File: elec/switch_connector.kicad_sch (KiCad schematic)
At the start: 7 parts, among them J3 BM04B-SRSS-TB, Q1 2N7002

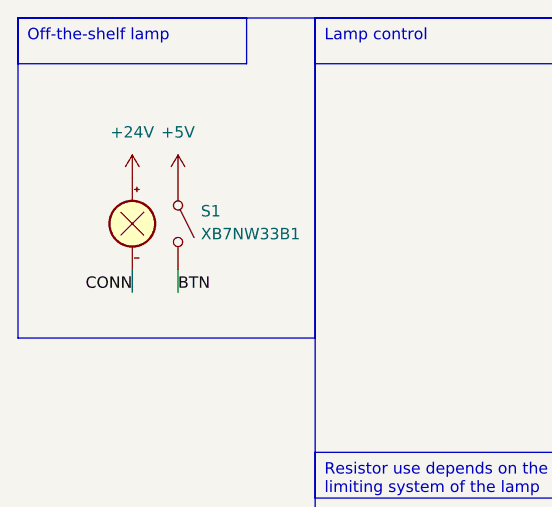
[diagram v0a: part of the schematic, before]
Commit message: dev: updating pcb
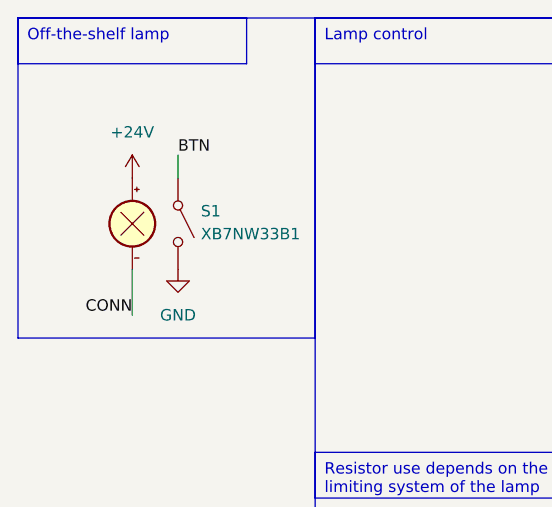
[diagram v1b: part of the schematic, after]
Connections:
- net +5V is gone; now on net BTN: S1.1 (13)
- net BTN: no longer S1.2 (14)
- net GND: now also S1.2 (14)
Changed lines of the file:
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@@
 	(wire
 		(pts
-			(xy 25.4 43.18) (xy 25.4 40.64)
+			(xy 25.4 45.72) (xy 25.4 40.64)
 		)
 		(stroke
@@
 	(wire
 		(pts
-			(xy 30.48 43.18) (xy 30.48 40.64)
+			(xy 30.48 27.94) (xy 30.48 30.48)
 		)
 		(stroke
@@
 	)
 	(label "BTN"
-		(at 30.48 43.18 0)
+		(at 30.48 27.94 0)
 		(fields_autoplaced yes)
 		(effects
@@
 	)
 	(label "CONN"
-		(at 25.4 43.18 180)
+		(at 25.4 45.72 180)
 		(fields_autoplaced yes)
 		(effects
@@
 	)
 	(symbol
+		(lib_id "power:GND")
+		(at 30.48 40.64 0)
+		(unit 1)
+		(exclude_from_sim no)
+		(in_bom yes)
+		(on_board yes)
+		(dnp no)
+		(fields_autoplaced yes)
+		(property "Reference" "#PWR028"
+			(at 30.48 46.99 0)
+			(effects
+				(font
+					(size 1.27 1.27)
+				)
+				(hide yes)
+			)
+		)
+		(property "Value" "GND"
+			(at 30.48 45.72 0)
+			(effects
+				(font
+					(size 1.27 1.27)
+				)
+			)
+		)
+		(property "Footprint" ""
+			(at 30.48 40.64 0)
+			(effects
+				(font
+					(size 1.27 1.27)
+				)
+				(hide yes)
+			)
+		)
+		(property "Datasheet" ""
+			(at 30.48 40.64 0)
+			(effects
+				(font
+					(size 1.27 1.27)
+				)
+				(hide yes)
+			)
+		)
+		(property "Description" "Power symbol creates a global label with name \"GND\" , ground"
+			(at 30.48 40.64 0)
+			(effects
+				(font
+					(size 1.27 1.27)
+				)
+				(hide yes)
+			)
+		)
+		(pin "1"
+		)
+		(instances
+			(project "elec"
+				(path "/9721bce9-01f4-4230-bc1e-748d0303b61d/d1c63f12-a9c6-44fc-aada-0b6e04e33293"
+					(reference "#PWR028")
+					(unit 1)
+				)
+				(path "/9721bce9-01f4-4230-bc1e-748d0303b61d/5ed1a42c-1f8a-456f-aca4-b0ec53e5043f"
+					(reference "#PWR036")
+					(unit 1)
+				)
+				(path "/9721bce9-01f4-4230-bc1e-748d0303b61d/fdf19939-3d9b-4110-9022-c37157a29402"
+					(reference "#PWR044")
+					(unit 1)
+				)
+				(path "/9721bce9-01f4-4230-bc1e-748d0303b61d/37f927af-89ef-4fdd-8956-bca34548d96f"
+					(reference "#PWR052")
+					(unit 1)
+				)
+				(path "/9721bce9-01f4-4230-bc1e-748d0303b61d/986b1860-5bd6-47a5-b66e-b737b7bd0f11"
+					(reference "#PWR060")
+					(unit 1)
+				)
+				(path "/9721bce9-01f4-4230-bc1e-748d0303b61d/eebd9391-916f-49b6-bec7-88d6969a1573"
+					(reference "#PWR068")
+					(unit 1)
+				)
+				(path "/9721bce9-01f4-4230-bc1e-748d0303b61d/d67cbc77-a7b3-4445-bb70-2db77a7feb74"
+					(reference "#PWR076")
+					(unit 1)
+				)
+				(path "/9721bce9-01f4-4230-bc1e-748d0303b61d/3bc99195-9e3c-4290-911f-d629015a354c"
+					(reference "#PWR084")
+					(unit 1)
+				)
+				(path "/9721bce9-01f4-4230-bc1e-748d0303b61d/e3e2ca04-3651-46d9-8ec0-5b3aca5c73d2"
+					(reference "#PWR092")
+					(unit 1)
+				)
+				(path "/9721bce9-01f4-4230-bc1e-748d0303b61d/333f48b8-09d6-4cfc-b48e-393e968338e9"
+					(reference "#PWR0100")
+					(unit 1)
+				)
+			)
+		)
+	)
+	(symbol
 		(lib_id "breakout:XB7NW33B1")
 		(at 30.48 35.56 0)
@@
 					(unit 1)
 				)
-			)
-		)
-	)
-	(symbol
-		(lib_id "power:+5V")
-		(at 30.48 30.48 0)
-		(unit 1)
-		(exclude_from_sim no)
-		(in_bom yes)
-		(on_board yes)
-		(dnp no)
-		(fields_autoplaced yes)
-		(property "Reference" "#PWR028"
-			(at 30.48 34.29 0)
-			(effects
-				(font
-					(size 1.27 1.27)
-				)
-				(hide yes)
-			)
-		)
-		(property "Value" "+5V"
-			(at 30.48 25.4 0)
-			(effects
-				(font
-					(size 1.27 1.27)
-				)
-			)
-		)
-		(property "Footprint" ""
-			(at 30.48 30.48 0)
-			(effects
-				(font
-					(size 1.27 1.27)
-				)
-				(hide yes)
-			)
-		)
-		(property "Datasheet" ""
-			(at 30.48 30.48 0)
-			(effects
-				(font
-					(size 1.27 1.27)
-				)
-				(hide yes)
-			)
-		)
-		(property "Description" "Power symbol creates a global label with name \"+5V\""
-			(at 30.48 30.48 0)
-			(effects
-				(font
-					(size 1.27 1.27)
-				)
-				(hide yes)
-			)
-		)
-		(pin "1"
-		)
-		(instances
-			(project "elec"
-				(path "/9721bce9-01f4-4230-bc1e-748d0303b61d/d1c63f12-a9c6-44fc-aada-0b6e04e33293"
-					(reference "#PWR028")
-					(unit 1)
-				)
-				(path "/9721bce9-01f4-4230-bc1e-748d0303b61d/5ed1a42c-1f8a-456f-aca4-b0ec53e5043f"
-					(reference "#PWR036")
-					(unit 1)
-				)
-				(path "/9721bce9-01f4-4230-bc1e-748d0303b61d/fdf19939-3d9b-4110-9022-c37157a29402"
-					(reference "#PWR044")
-					(unit 1)
-				)
-				(path "/9721bce9-01f4-4230-bc1e-748d0303b61d/37f927af-89ef-4fdd-8956-bca34548d96f"
-					(reference "#PWR052")
-					(unit 1)
-				)
-				(path "/9721bce9-01f4-4230-bc1e-748d0303b61d/986b1860-5bd6-47a5-b66e-b737b7bd0f11"
-					(reference "#PWR060")
-					(unit 1)
-				)
-				(path "/9721bce9-01f4-4230-bc1e-748d0303b61d/eebd9391-916f-49b6-bec7-88d6969a1573"
-					(reference "#PWR068")
-					(unit 1)
-				)
-				(path "/9721bce9-01f4-4230-bc1e-748d0303b61d/d67cbc77-a7b3-4445-bb70-2db77a7feb74"
-					(reference "#PWR076")
-					(unit 1)
-				)
-				(path "/9721bce9-01f4-4230-bc1e-748d0303b61d/3bc99195-9e3c-4290-911f-d629015a354c"
-					(reference "#PWR084")
-					(unit 1)
-				)
-				(path "/9721bce9-01f4-4230-bc1e-748d0303b61d/e3e2ca04-3651-46d9-8ec0-5b3aca5c73d2"
-					(reference "#PWR092")
-					(unit 1)
-				)
-				(path "/9721bce9-01f4-4230-bc1e-748d0303b61d/333f48b8-09d6-4cfc-b48e-393e968338e9"
-					(reference "#PWR0100")
-					(unit 1)
-				)
